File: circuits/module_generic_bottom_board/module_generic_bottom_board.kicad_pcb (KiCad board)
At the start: 2 copper layers, 24.1 x 77.5 mm, 7 parts, among them P1 CONN_02X05, P2 CONN_02X05, P3 CONN_01X11, P4 CONN_01X01, P5 CONN_01X01

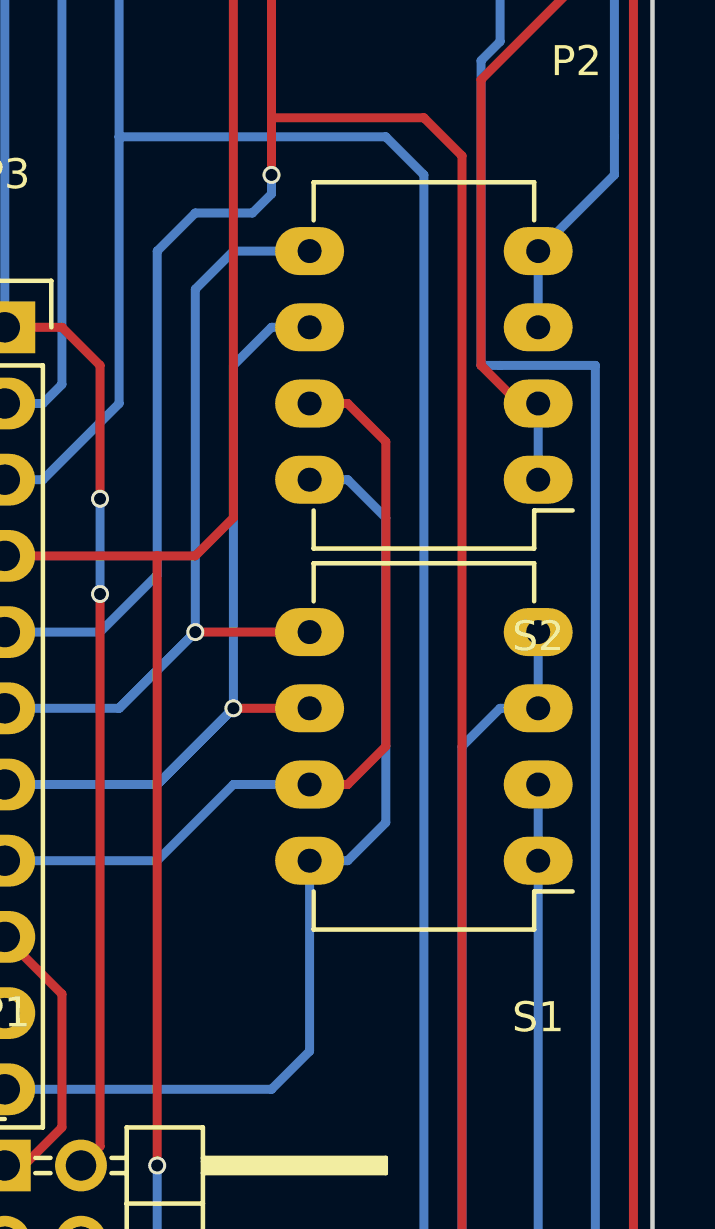
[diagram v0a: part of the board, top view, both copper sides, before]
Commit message: Update circuits
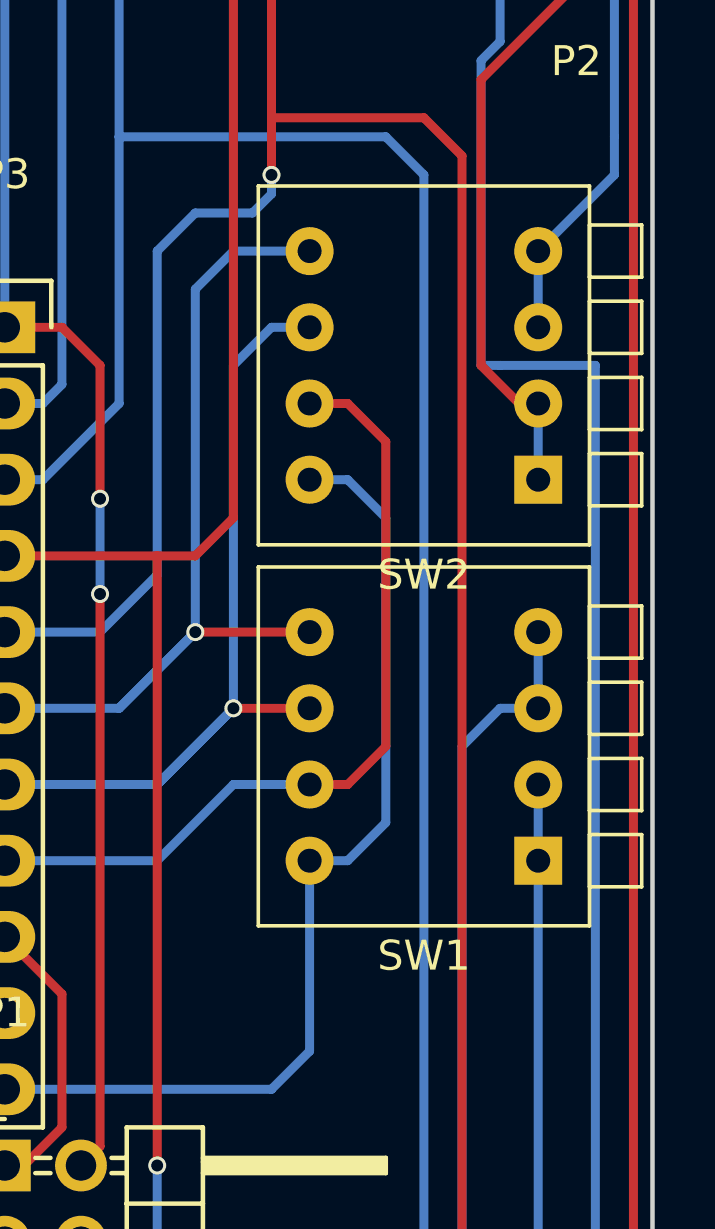
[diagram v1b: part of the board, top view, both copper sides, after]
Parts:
- removed S1, S2: SW_DIP_x4, Housings_DIP:DIP-8_W7.62mm_LongPads
- added SW1: SW_DIP_x04, Buttons_Switches_THT:SW_DIP_x4_W7.62mm_Piano, F.Cu at (154.9, 132.1)
- added SW2: SW_DIP_x04, Buttons_Switches_THT:SW_DIP_x4_W7.62mm_Piano, F.Cu at (154.9, 119.4)
